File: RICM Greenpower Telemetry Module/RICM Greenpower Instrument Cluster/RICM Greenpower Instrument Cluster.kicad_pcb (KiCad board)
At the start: 2 copper layers, 110 x 43.2 mm, 16 parts, among them J1 Conn_02x04_Counter_Clockwise, SW1 SW_Push, SW2 SW_Push, U1 PCA9555D

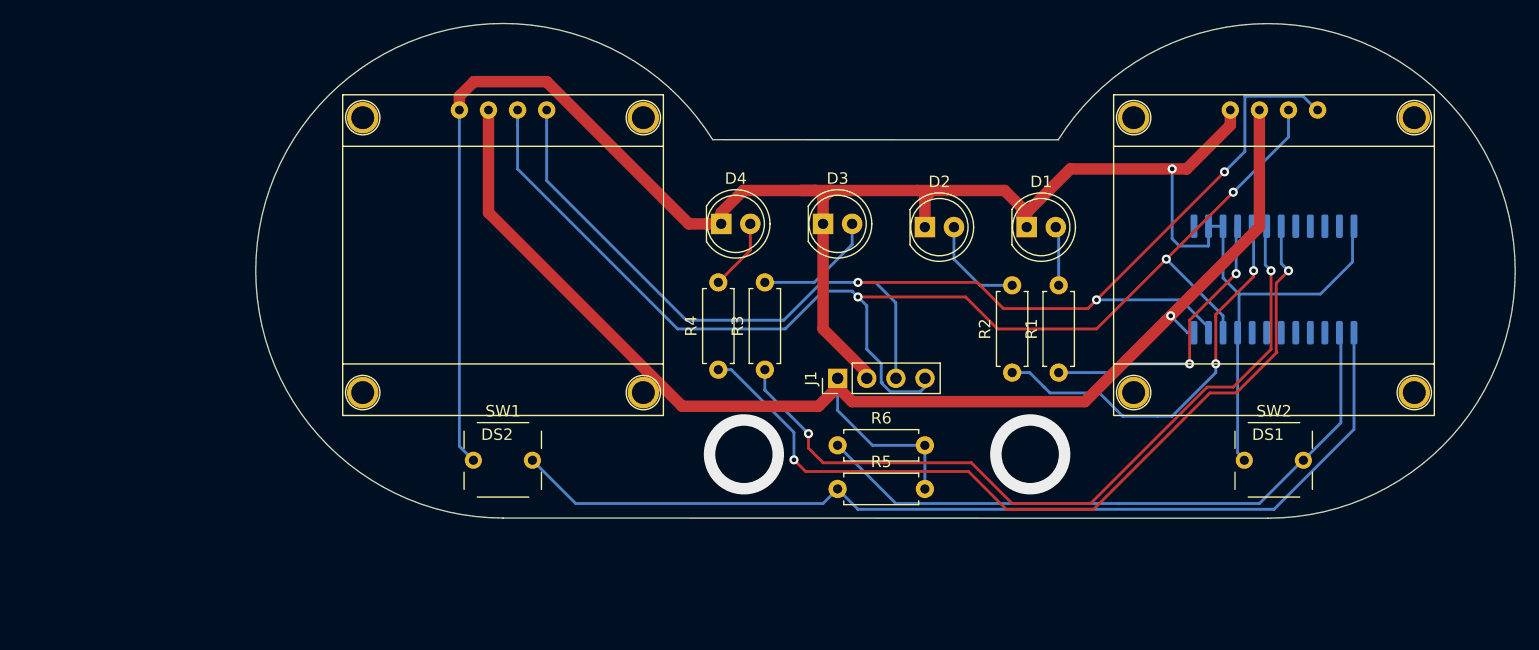
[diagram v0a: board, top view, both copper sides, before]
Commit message: last revisions before first order
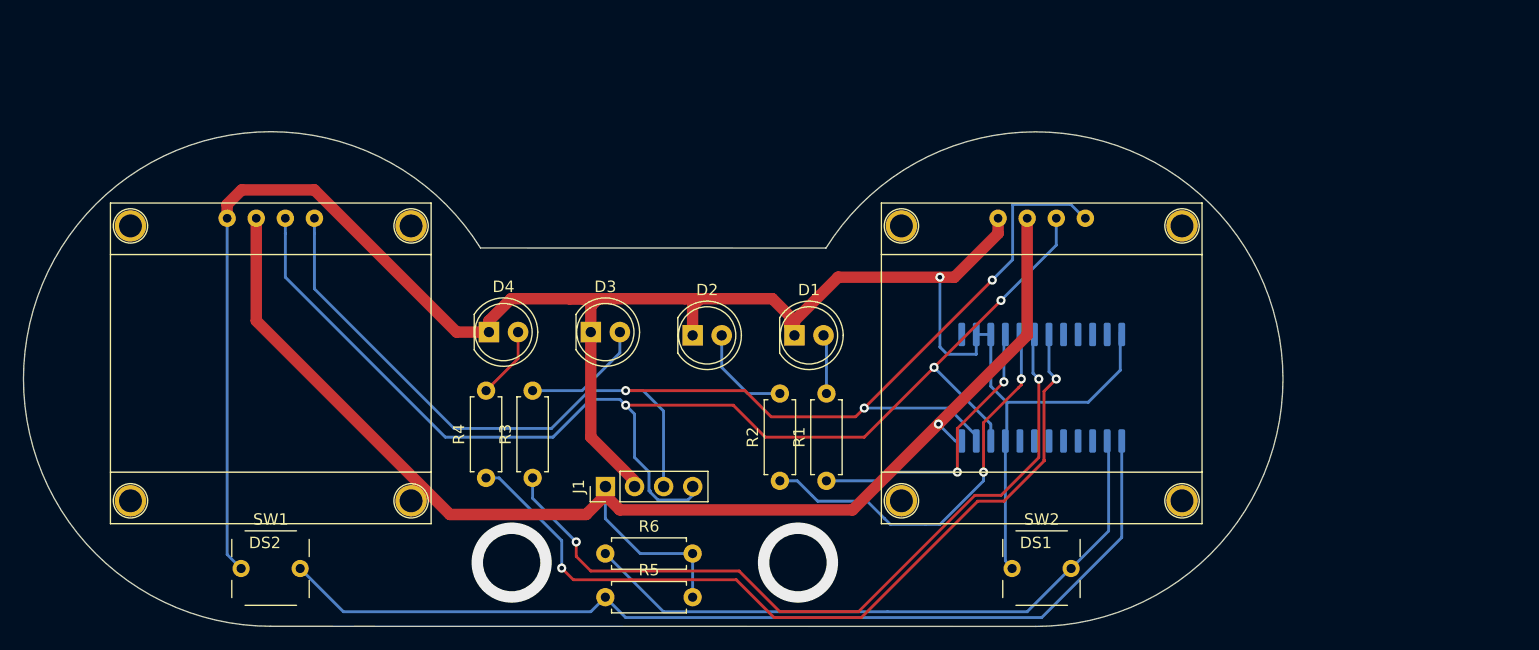
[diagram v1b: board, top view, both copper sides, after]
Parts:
- moved J1 22.4 mm to (22.9, 32.8)
- moved D4 22.4 mm to (12.7, 19.3)
- moved DS1 22.4 mm to (61.0, 36.1)
- moved DS2 22.4 mm to (-6.31, 36.1)
- moved R1 22.4 mm to (42.2, 32.3)
- moved R2 22.4 mm to (38.1, 32.3)
- moved SW1 22.4 mm to (-9.56, 37.7)
- moved SW2 22.4 mm to (57.8, 37.7)
- moved U1 22.4 mm to (61.0, 24.2)
- moved D2 22.4 mm to (30.5, 19.6)
- moved D3 22.4 mm to (21.6, 19.3)
- moved R3 22.4 mm to (16.6, 32.1)
- moved R4 22.4 mm to (12.5, 32.1)
- moved R5 22.4 mm to (22.9, 42.5)
- moved R6 22.4 mm to (22.9, 38.7)
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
